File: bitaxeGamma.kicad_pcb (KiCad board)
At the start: 4 copper layers, 56.5 x 99.8 mm, 146 parts, among them J1 54-00164, J2 TC2030-IDC, J3 Conn_01x04, J4 Conn_01x06, J5 USB_C_Receptacle_USB2.0, J6 Conn_01x04, J7 Conn_01x04, SW1 GT-TC029B-H025-L1N, SW2 GT-TC029B-H025-L1N, T1 net-tie, U10 EMC2101, U2 TPS546D24ARVFR, U3 RT9080-33GJ5, U4 ESP32-S3-WROOM-1, U5 MCP1824T-1202E/OT, U6 MCP1824T-0802E, U7 25MHz, U8 BM1370_mode1, U9 SN74AVC4T774

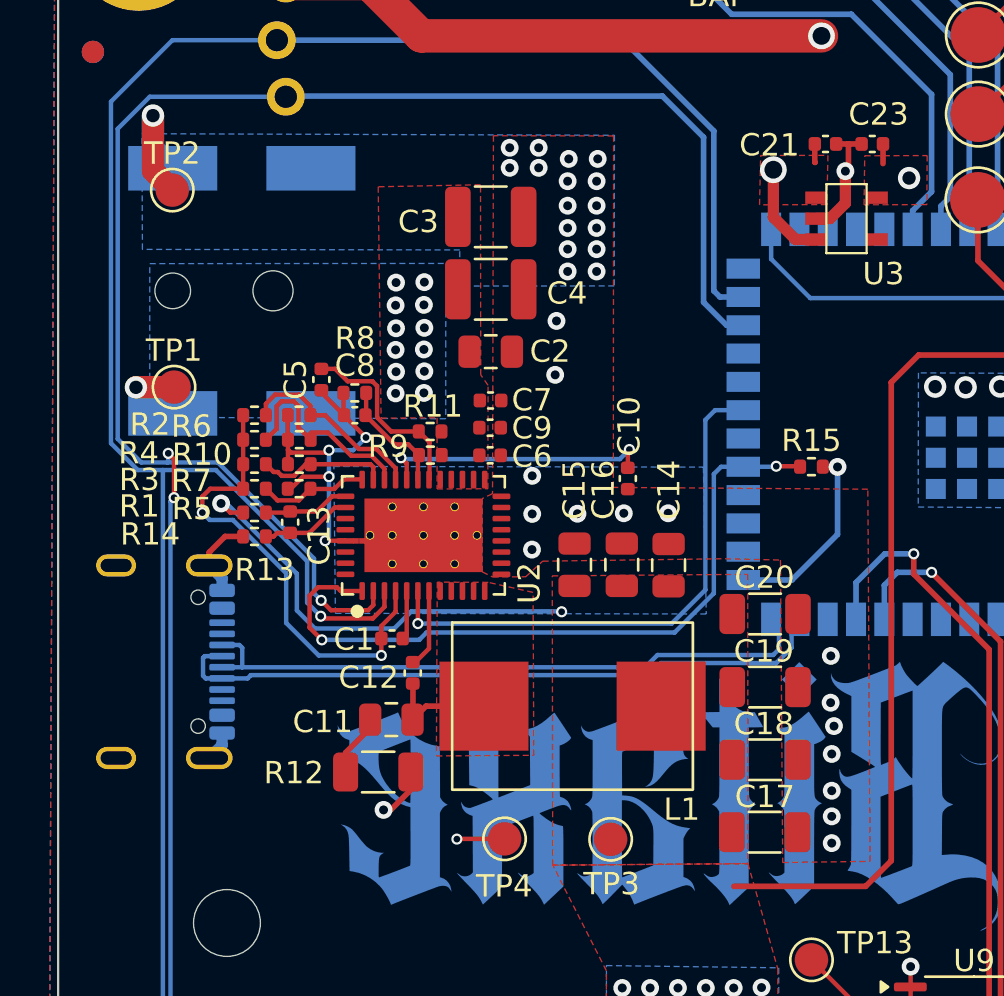
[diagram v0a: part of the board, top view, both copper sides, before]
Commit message: fix zones...
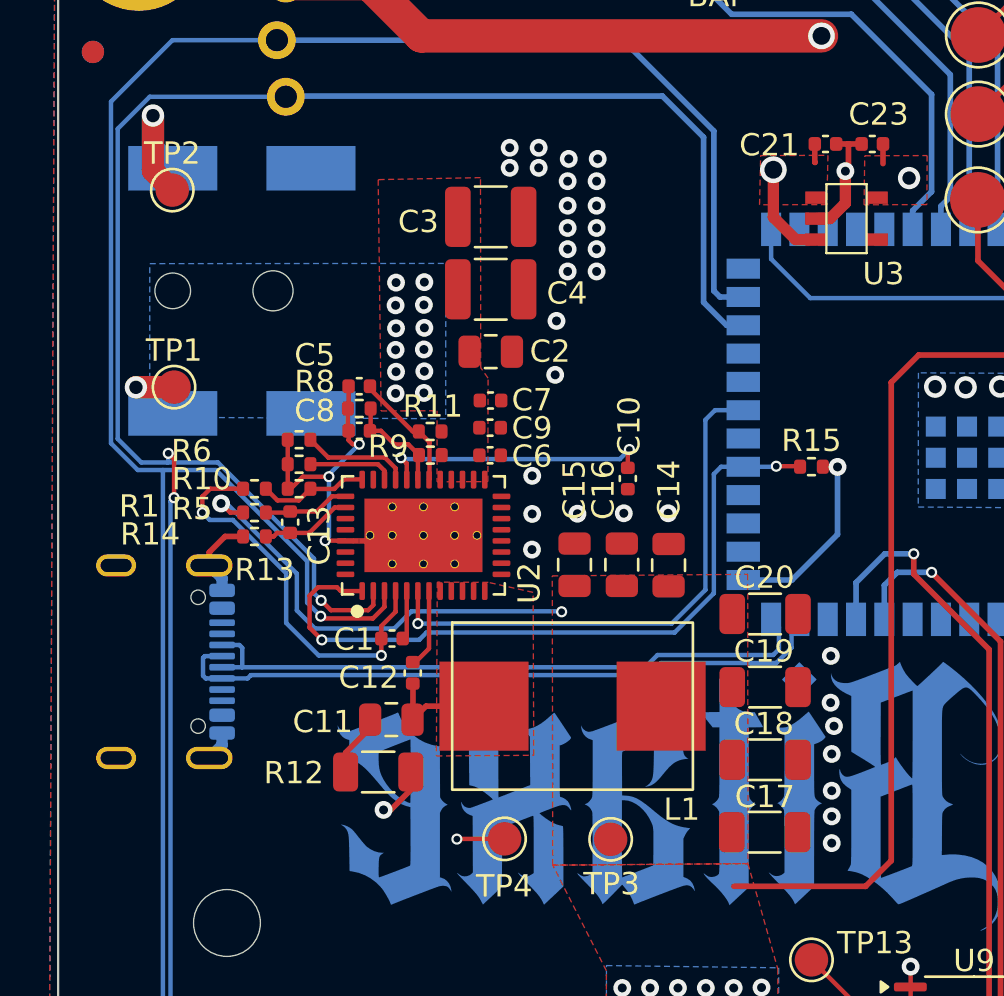
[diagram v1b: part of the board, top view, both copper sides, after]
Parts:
- removed R2, R3, R4, R7: ~, Resistor_SMD:R_0402_1005Metric
- moved C5 1.73 mm to (90.7, 70.9), turned to 0 degrees
- moved R10 1.10 mm to (88.0, 74.4)
- moved R6 1.10 mm to (88.0, 73.3)
- moved C8 0.73 mm to (90.7, 72.9)
- moved R8 0.73 mm to (90.7, 71.9)
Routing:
- net Net-(U2-ADRSEL): track 5.87 -> 0.00 mm
- net Net-(U2-VSEL): track 9.06 -> 3.84 mm
- net /Power/AGND: track 17.1 -> 13.2 mm, vias 4 -> 3
- net Net-(U2-MSEL2): track 8.63 -> 4.86 mm
- net Net-(U2-BP1V5): track 21.1 -> 17.8 mm
- net Net-(U2-AVIN): track 8.73 -> 5.46 mm
